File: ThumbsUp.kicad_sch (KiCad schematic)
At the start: 58 parts, among them J1 52559-1233, J1L1 PJ-3200B, J1R1 PJ-3200B, J2 52559-1233, U1 ProMicro

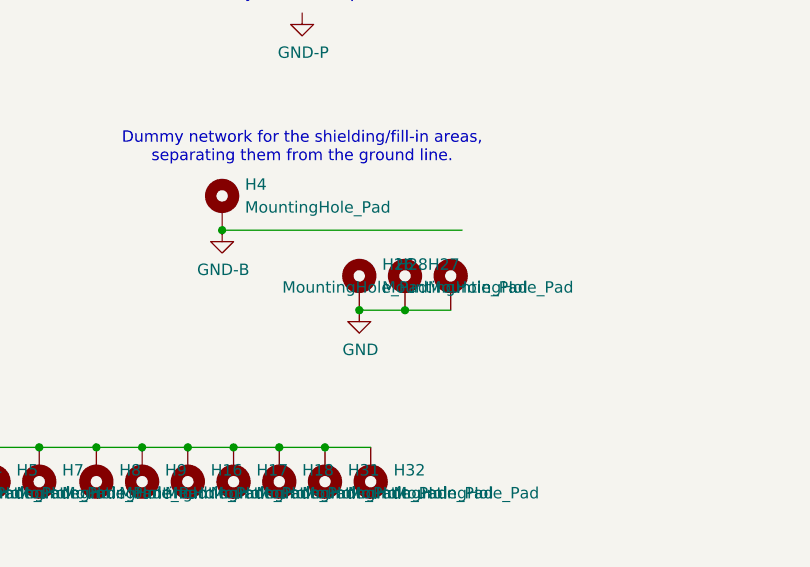
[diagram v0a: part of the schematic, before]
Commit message: v12: Minor corrections.
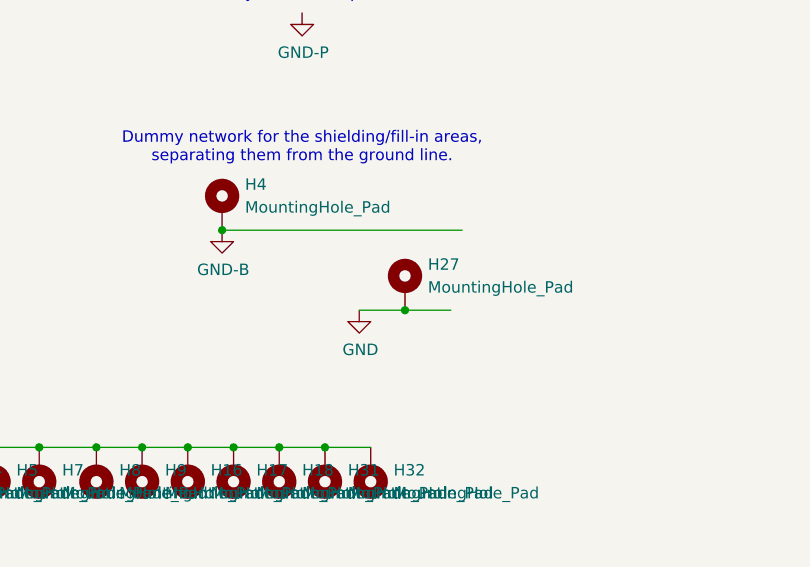
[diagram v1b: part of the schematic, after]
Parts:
- removed H26, H28: MountingHole_Pad, MountingHole:MountingHole_4.5mm_Pad, symbol Mechanical:MountingHole_Pad
- H27: footprint MountingHole:MountingHole_4.5mm_Pad -> MountingHole:MountingHole_3.5mm_Pad
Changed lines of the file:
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@@
 	)
 	(junction
-		(at 477.52 262.89)
-		(diameter 0)
-		(color 0 0 0 0)
-	)
-	(junction
 		(at 438.15 207.01)
 		(diameter 0)
@@
 	(symbol
 		(lib_id "Mechanical:MountingHole_Pad")
-		(at 487.68 260.35 0)
-		(mirror y)
-		(unit 1)
-		(exclude_from_sim no)
-		(in_bom no)
-		(on_board yes)
-		(dnp no)
-		(property "Reference" "H28"
-			(at 485.14 257.8099 0)
-			(effects
-				(font
-					(size 1.27 1.27)
-				)
-				(justify left)
-			)
-		)
-		(property "Value" "MountingHole_Pad"
-			(at 485.14 260.3499 0)
-			(effects
-				(font
-					(size 1.27 1.27)
-				)
-				(justify left)
-			)
-		)
-		(property "Footprint" "MountingHole:MountingHole_4.5mm_Pad"
-			(at 487.68 260.35 0)
-			(effects
-				(font
-					(size 1.27 1.27)
-				)
-				(hide yes)
-			)
-		)
-		(property "Datasheet" "~"
-			(at 487.68 260.35 0)
-			(effects
-				(font
-					(size 1.27 1.27)
-				)
-				(hide yes)
-			)
-		)
-		(property "Description" "Mounting Hole with connection"
-			(at 487.68 260.35 0)
-			(effects
-				(font
-					(size 1.27 1.27)
-				)
-				(hide yes)
-			)
-		)
-		(pin "1"
-		)
-		(instances
-			(project "ThumbsUp"
-				(path "/467ed76c-995a-4514-a2e9-81ed0f98430e"
-					(reference "H28")
-					(unit 1)
-				)
-			)
-		)
-	)
-	(symbol
-		(lib_id "Mechanical:MountingHole_Pad")
 		(at 436.88 280.67 180)
 		(unit 1)
@@
 	(symbol
 		(lib_id "Mechanical:MountingHole_Pad")
-		(at 477.52 260.35 0)
-		(unit 1)
-		(exclude_from_sim no)
-		(in_bom no)
-		(on_board yes)
-		(dnp no)
-		(fields_autoplaced yes)
-		(property "Reference" "H26"
-			(at 480.06 257.8099 0)
-			(effects
-				(font
-					(size 1.27 1.27)
-				)
-				(justify left)
-			)
-		)
-		(property "Value" "MountingHole_Pad"
-			(at 480.06 260.3499 0)
-			(effects
-				(font
-					(size 1.27 1.27)
-				)
-				(justify left)
-			)
-		)
-		(property "Footprint" "MountingHole:MountingHole_4.5mm_Pad"
-			(at 477.52 260.35 0)
-			(effects
-				(font
-					(size 1.27 1.27)
-				)
-				(hide yes)
-			)
-		)
-		(property "Datasheet" "~"
-			(at 477.52 260.35 0)
-			(effects
-				(font
-					(size 1.27 1.27)
-				)
-				(hide yes)
-			)
-		)
-		(property "Description" "Mounting Hole with connection"
-			(at 477.52 260.35 0)
-			(effects
-				(font
-					(size 1.27 1.27)
-				)
-				(hide yes)
-			)
-		)
-		(pin "1"
-		)
-		(instances
-			(project "ThumbsUp"
-				(path "/467ed76c-995a-4514-a2e9-81ed0f98430e"
-					(reference "H26")
-					(unit 1)
-				)
-			)
-		)
-	)
-	(symbol
-		(lib_id "Mechanical:MountingHole_Pad")
 		(at 420.37 309.88 0)
 		(unit 1)
@@
 			)
 		)
-		(property "Footprint" "MountingHole:MountingHole_4.5mm_Pad"
+		(property "Footprint" "MountingHole:MountingHole_3.5mm_Pad"
 			(at 482.6 260.35 0)
 			(effects
